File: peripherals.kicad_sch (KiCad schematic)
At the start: 75 parts, among them J1 USB-C_USB4105-GF-A, J10 PinHeader_1x6_P2.54mm_SMD_Hor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, J4 Conn_FFC_WE_68715014522_ONE-S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, J5 PinHeader_2x5_P1.27mm_SMD, J6 Conn_FFC_WE_68715014522_ONE-S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, J8 SM04B-SRSS-TB-LF-SN, J9 SM06B-GHS-TB-LF-SN, SW1 SW_CVS-02B, U11 LIFCL-40-9BG256C, U13 DIO7553ST6, U14 DIO7553ST6, U19 DIO7553ST6, U20 FT230X_QFN

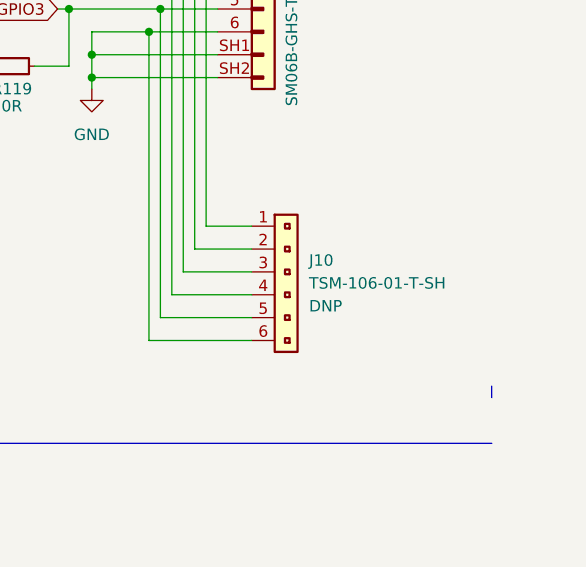
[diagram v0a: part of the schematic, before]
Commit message: [#55653] Update TSM-106-01-T-SH
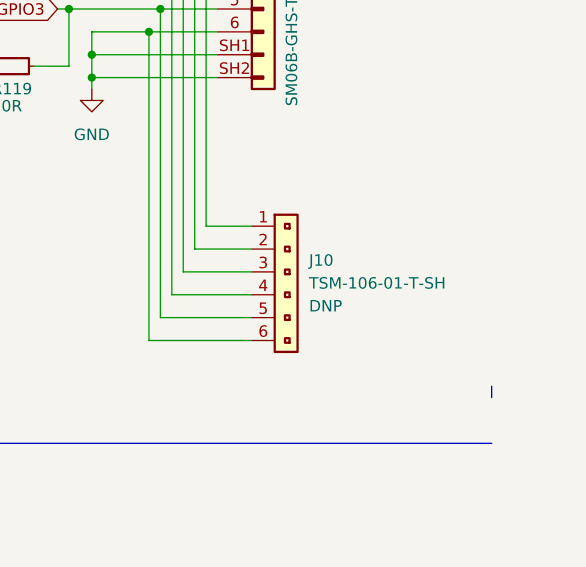
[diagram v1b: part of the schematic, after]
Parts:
- J10: footprint sdi-mipi-video-converter-footprints:PinHeader_1x6_TSM-106-01-T-SH -> antmicro-footprints:PinHeader_1x6_P2.54mm_SMD_Horizontal; symbol sdi-mipi-video-converter:PinHeader_1x6_P2.54mm_SMD_Horizontal -> antmicroGenericPinHeaders:PinHeader_1x6_P2.54mm_SMD_Horizontal
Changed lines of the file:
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@@
     )
   )
-  (symbol (lib_id "sdi-mipi-video-converter:PinHeader_1x6_P2.54mm_SMD_Horizontal") (at 381 69.85 0) (unit 1)
+  (symbol (lib_id "antmicroGenericPinHeaders:PinHeader_1x6_P2.54mm_SMD_Horizontal") (at 381 69.85 0) (unit 1)
     (in_bom yes) (on_board yes) (dnp no) (fields_autoplaced)
-    (property "Reference" "J10" (at 387.35 73.6599 0)
+    (property "Reference" "J10" (at 387.35 73.66 0)
       (effects (font (size 1.27 1.27) (thickness 0.15)) (justify left))
     )
@@
       (effects (font (size 1.27 1.27) (thickness 0.15)) (justify left bottom) hide)
     )
-    (property "Footprint" "sdi-mipi-video-converter-footprints:PinHeader_1x6_TSM-106-01-T-SH" (at 400.05 81.28 0)
+    (property "Footprint" "antmicro-footprints:PinHeader_1x6_P2.54mm_SMD_Horizontal" (at 400.05 81.28 0)
       (effects (font (size 1.27 1.27) (thickness 0.15)) (justify left bottom) hide)
     )
-    (property "Datasheet" "https://www.mouser.pl/datasheet/2/527/tsm-2854655.pdf" (at 400.05 83.82 0)
+    (property "Datasheet" "https://www.mouser.com/datasheet/2/527/tsm-2854655.pdf" (at 400.05 83.82 0)
       (effects (font (size 1.27 1.27) (thickness 0.15)) (justify left bottom) hide)
     )
@@
       (effects (font (size 1.27 1.27) (thickness 0.15)) (justify left bottom) hide)
     )
-    (property "MPN" "TSM-106-01-T-SH" (at 387.35 76.1999 0)
+    (property "MPN" "TSM-106-01-T-SH" (at 387.35 76.2 0)
       (effects (font (size 1.27 1.27) (thickness 0.15)) (justify left))
     )
@@
       (effects (font (size 1.27 1.27) (thickness 0.15)) (justify left bottom) hide)
     )
-    (property "DNP" "DNP" (at 387.35 78.7399 0)
+    (property "DNP" "DNP" (at 387.35 78.74 0)
       (effects (font (size 1.27 1.27)) (justify left))
     )
